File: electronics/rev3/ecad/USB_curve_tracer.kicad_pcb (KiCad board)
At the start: 2 copper layers, 117 x 64 mm, 66 parts, among them J1 DUT Connector, J2 Power Input, Q1 TIP122, Q2 TIP127, Q5 TIP122, Q6 TIP127, U1 MCP4911, U2 LMC6484IN, U3 MCP3204, U4 LM385BZ-2.5

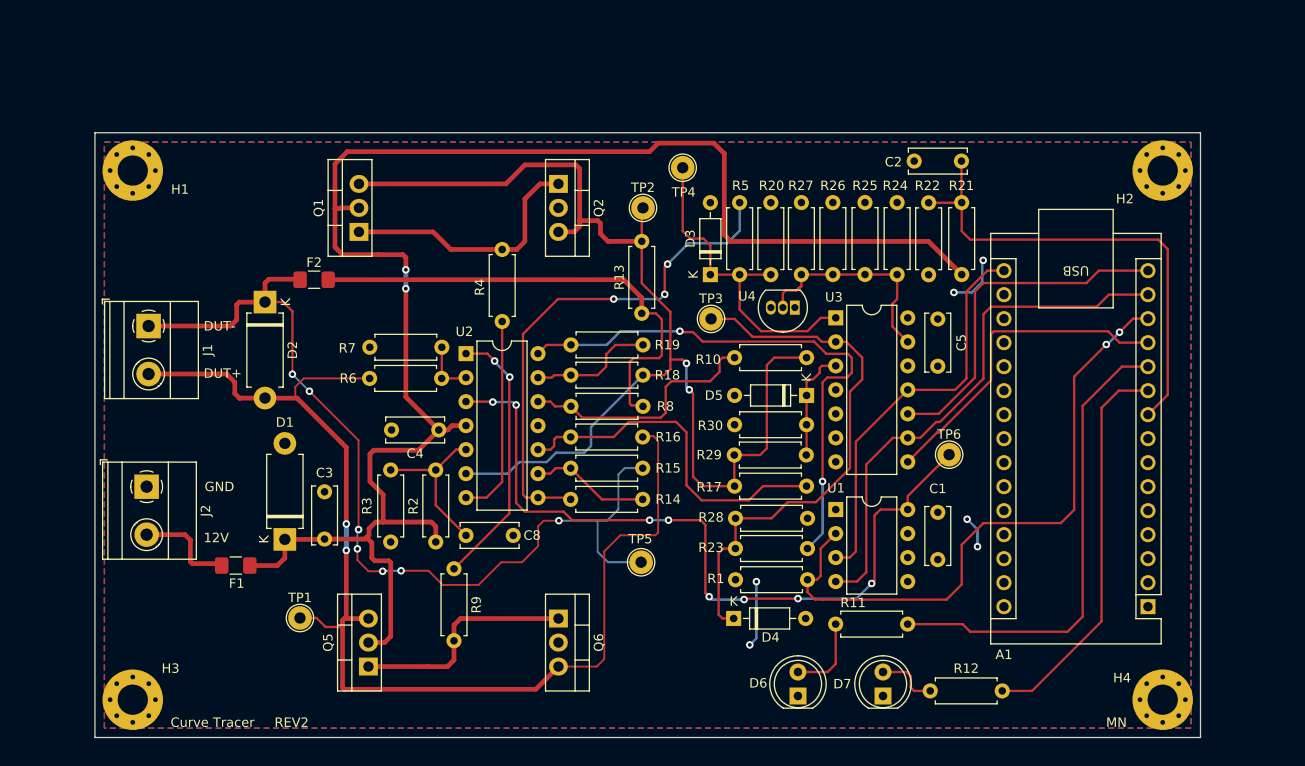
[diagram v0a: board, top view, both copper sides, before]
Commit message: Layout work
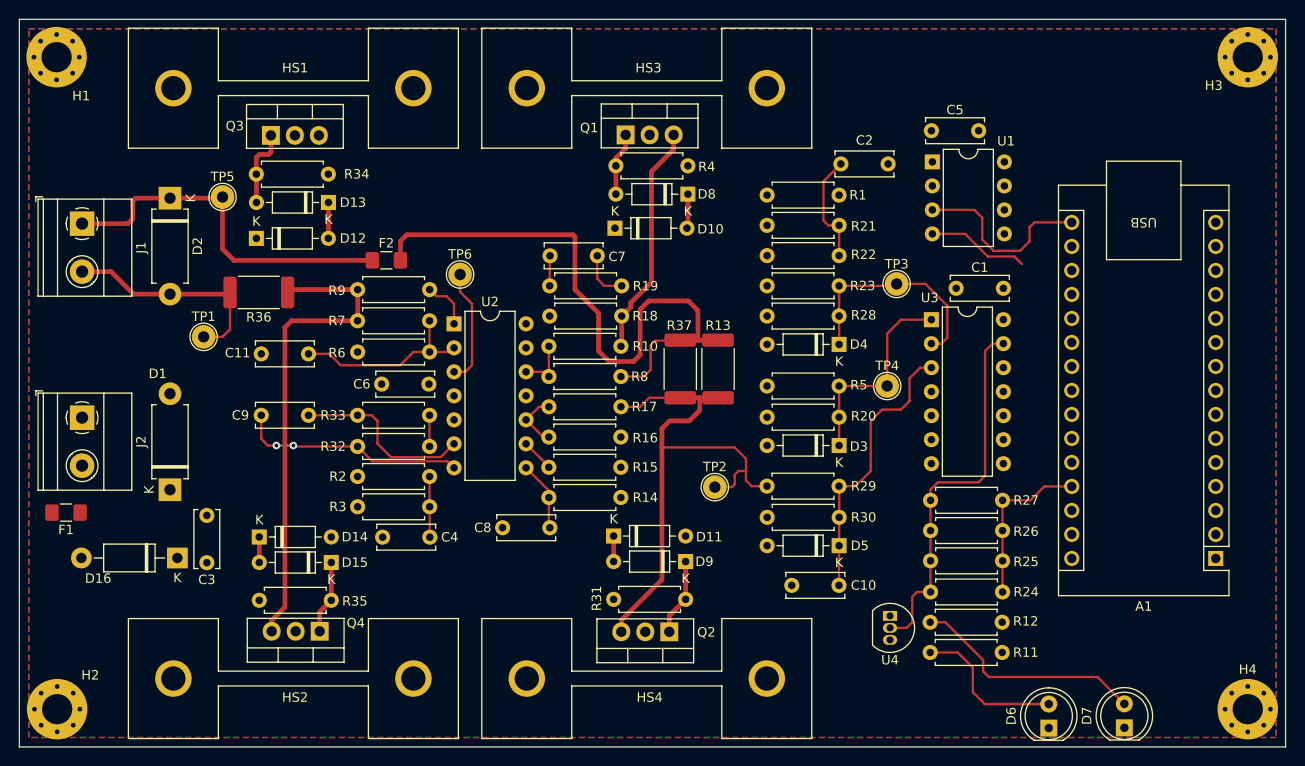
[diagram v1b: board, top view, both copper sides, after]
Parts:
- removed Q5: TIP122, Package_TO_SOT_THT:TO-220-3_Vertical
- removed Q6: TIP127, Package_TO_SOT_THT:TO-220-3_Vertical
- added C10: 0.1uF, Capacitor_THT:C_Disc_D6.0mm_W2.5mm_P5.00mm, F.Cu at (161.7, 116.9)
- added C11: 100pF, Capacitor_THT:C_Disc_D6.0mm_W2.5mm_P5.00mm, F.Cu at (100.6, 92.4)
- added C6: 0.1uF, Capacitor_THT:C_Disc_D6.0mm_W2.5mm_P5.00mm, F.Cu at (118.3, 95.6)
- added C7: 10nF, Capacitor_THT:C_Disc_D6.0mm_W2.5mm_P5.00mm, F.Cu at (136.2, 82.0)
- added C9: 100pF, Capacitor_THT:C_Disc_D6.0mm_W2.5mm_P5.00mm, F.Cu at (105.6, 98.9)
- added D10: 1N4148, Diode_THT:D_DO-35_SOD27_P7.62mm_Horizontal, F.Cu at (138.0, 79.1)
- added D11: 1N4148, Diode_THT:D_DO-35_SOD27_P7.62mm_Horizontal, F.Cu at (137.9, 111.7)
- added D12: 1N4148, Diode_THT:D_DO-35_SOD27_P7.62mm_Horizontal, F.Cu at (100.1, 80.2)
- added D13: 1N4148, Diode_THT:D_DO-35_SOD27_P7.62mm_Horizontal, F.Cu at (107.7, 76.4)
- added D14: 1N4148, Diode_THT:D_DO-35_SOD27_P7.62mm_Horizontal, F.Cu at (100.4, 111.8)
- added D15: 1N4148, Diode_THT:D_DO-35_SOD27_P7.62mm_Horizontal, F.Cu at (108.0, 114.5)
- added D16: 1N5817, Diode_THT:D_DO-41_SOD81_P10.16mm_Horizontal, F.Cu at (91.7, 114.0)
- added D8: 1N4148, Diode_THT:D_DO-35_SOD27_P7.62mm_Horizontal, F.Cu at (145.8, 75.5)
- added D9: 1N4148, Diode_THT:D_DO-35_SOD27_P7.62mm_Horizontal, F.Cu at (145.5, 114.4)
- added HS1: 13.40°C/W, Library:HSINK_531002B02500G, F.Cu at (104.0, 64.3)
- added HS2: 13.40°C/W, Library:HSINK_531002B02500G, F.Cu at (104.0, 126.8)
- added HS3: 13.40°C/W, Library:HSINK_531002B02500G, F.Cu at (141.4, 64.3)
- added HS4: 13.40°C/W, Library:HSINK_531002B02500G, F.Cu at (141.4, 126.8)
- added Q3: TIP122, Package_TO_SOT_THT:TO-220-3_Vertical, F.Cu at (101.6, 69.3)
- added Q4: TIP127, Package_TO_SOT_THT:TO-220-3_Vertical, F.Cu at (106.8, 121.8)
- added R31: 4.7k, Resistor_THT:R_Axial_DIN0207_L6.3mm_D2.5mm_P7.62mm_Horizontal, F.Cu at (145.5, 118.4)
- added R32: 1k, Resistor_THT:R_Axial_DIN0207_L6.3mm_D2.5mm_P7.62mm_Horizontal, F.Cu at (110.8, 102.2)
- added R33: 10k, Resistor_THT:R_Axial_DIN0207_L6.3mm_D2.5mm_P7.62mm_Horizontal, F.Cu at (110.8, 98.9)
- added R34: 4.7k, Resistor_THT:R_Axial_DIN0207_L6.3mm_D2.5mm_P7.62mm_Horizontal, F.Cu at (107.7, 73.4)
- added R35: 4.7k, Resistor_THT:R_Axial_DIN0207_L6.3mm_D2.5mm_P7.62mm_Horizontal, F.Cu at (108.0, 118.5)
- added R36: 1.5, Resistor_SMD:R_2512_6332Metric_Pad1.40x3.35mm_HandSolder, F.Cu at (100.3, 85.9)
- added R37: 1+/-1%, Resistor_SMD:R_2512_6332Metric_Pad1.40x3.35mm_HandSolder, F.Cu at (144.9, 94.0)
- C8: value 0.1uF -> 10nF
- F1: value 2A -> 3A
- R10, R19: value 250k+/-0.1% -> 11.8k+/-0.1%
- R13: value 0.1+/-0.1% -> 1+/-1%; footprint Resistor_THT:R_Axial_DIN0207_L6.3mm_D2.5mm_P7.62mm_Horizontal -> Resistor_SMD:R_2512_6332Metric_Pad1.40x3.35mm_HandSolder
- R18, R8: value 10k+/-0.1% -> 1k+/-0.1%
- R20, R28: value 1k -> 1k+/-0.1%
- R23: value 3240 -> 3.83k+/-0.1%
- R29, R5: value 4.7k -> 3.83k+/-0.1%
- R4: value 1k -> 4.7k
- TP5, TP6: value TestPoint -> 4952
- U2: value LMC6484IN -> LMC6484A
- moved H3 136.2 mm to (205.0, 61.0)
- moved H2 130.1 mm to (79.0, 130.0)
- moved TP5 58.8 mm to (96.5, 75.8)
- moved TP6 55.2 mm to (121.6, 84.0)
- moved Q2 48.8 mm to (143.8, 121.8), turned to 180 degrees
- moved R24 42.7 mm to (179.1, 117.6), turned to 180 degrees
- moved R1 40.8 mm to (154.1, 75.6)
- moved R25 40.6 mm to (179.1, 114.3), turned to 180 degrees
- moved R26 39.1 mm to (179.1, 111.1), turned to 180 degrees
- moved U1 38.2 mm to (171.6, 72.1)
- moved R27 38.0 mm to (179.1, 107.9), turned to 180 degrees
- moved U4 34.1 mm to (167.1, 120.1), turned to -90 degrees
- moved TP4 31.7 mm to (166.8, 95.8)
- moved TP1 31.5 mm to (94.5, 90.6)
- moved D4 31.1 mm to (161.8, 91.4), turned to 180 degrees
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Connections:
- net /IV_Variation/DUT- renamed Net-(D2-A1)
- net /IV_Variation/VADJ renamed /IV_Variation/Sweep_Input
- C4 pad 1: +12V -> Net-(U2B-+)
- C8 pad 1: Net-(U2B-+) -> Net-(U2C--)
- C8 pad 2: GND -> Net-(C8-Pad2)
- D2 pad 2: /IV_Variation/DUT+ -> Net-(D2-A2)
- F1 pad 2: +12V -> Net-(D16-A)
- J1 pad 2: /IV_Variation/DUT+ -> Net-(D2-A2)
- Q1 pad 1: Net-(Q1-B) -> Net-(D8-A)
- Q2 pad 1: Net-(Q1-B) -> Net-(D9-K)
- R14 pad 2: Net-(R14-Pad2) -> Net-(C8-Pad2)
- R16 pad 1: /IV_Variation/DUT+ -> Net-(D2-A2)
- R4 pad 1: Net-(R4-Pad1) -> +12V
- R4 pad 2: Net-(Q1-B) -> Net-(D8-A)
- R5 pad 1: Net-(R14-Pad2) -> Net-(C8-Pad2)
- R6 pad 2: /IV_Variation/DUT+ -> GND
- R7 pad 2: GND -> /IV_Variation/Sweep Voltage Buffer/Sweep_Amplified
- R9 pad 2: Net-(Q5-B) -> /IV_Variation/Sweep Voltage Buffer/Sweep_Amplified
- TP1 pad 1: /IV_Variation/DUT+ -> Net-(D2-A2)
- U2 pad 6: V/2 -> Net-(U2B--)
- U2 pad 7: Net-(R4-Pad1) -> Net-(D10-K)
- U2 pad 8: Net-(R14-Pad2) -> Net-(C8-Pad2)
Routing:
- net +12V: track 176.2 -> 0.00 mm, vias 2 -> 0
- net /IV_Variation/DUT+: track 125.8 -> 0.00 mm, vias 2 -> 0
- net /IV_Variation/Sweep_Input: track 81.3 -> 12.3 mm, vias 8 -> 0
- net Net-(A1-D10): track 67.4 -> 0.00 mm, vias 2 -> 0
- net Net-(D2-A1): track 101.0 -> 39.0 mm, vias 7 -> 0
- net Net-(C7-Pad2): track 58.7 -> 3.20 mm, vias 2 -> 0
- net Net-(R14-Pad2): track 54.4 -> 0.00 mm, vias 3 -> 0
- net /IV_Variation/Sweep Voltage Buffer/Sweep_Amplified: track 0.00 -> 51.6 mm
- net Net-(A1-D8): track 50.4 -> 0.00 mm
- net Net-(A1-D11): track 56.3 -> 10.8 mm
- net Net-(A1-D7): track 41.8 -> 0.00 mm
- net Net-(A1-D6): track 51.9 -> 11.8 mm
- net V/2: track 126.0 -> 86.8 mm, vias 2 -> 0
- net Net-(A1-D12): track 37.0 -> 0.00 mm
- net Net-(A1-D9): track 34.5 -> 0.00 mm
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- added copper zone on F.Cu, net +12V
- removed copper zone on F.Cu, net +5V
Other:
- board size 117 x 64 mm -> 134 x 77 mm
- board text removed: "12V"
- board text removed: "Curve Tracer"
- board text removed: "DUT+"
- board text removed: "DUT-"
- board text removed: "GND"
- board text removed: "MN"
- board text removed: "REV2"
